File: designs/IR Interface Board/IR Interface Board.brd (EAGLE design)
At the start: 75 x 75 mm, 73 parts, among them IC1 REG1117, IC2 PIC16F1517/19PT

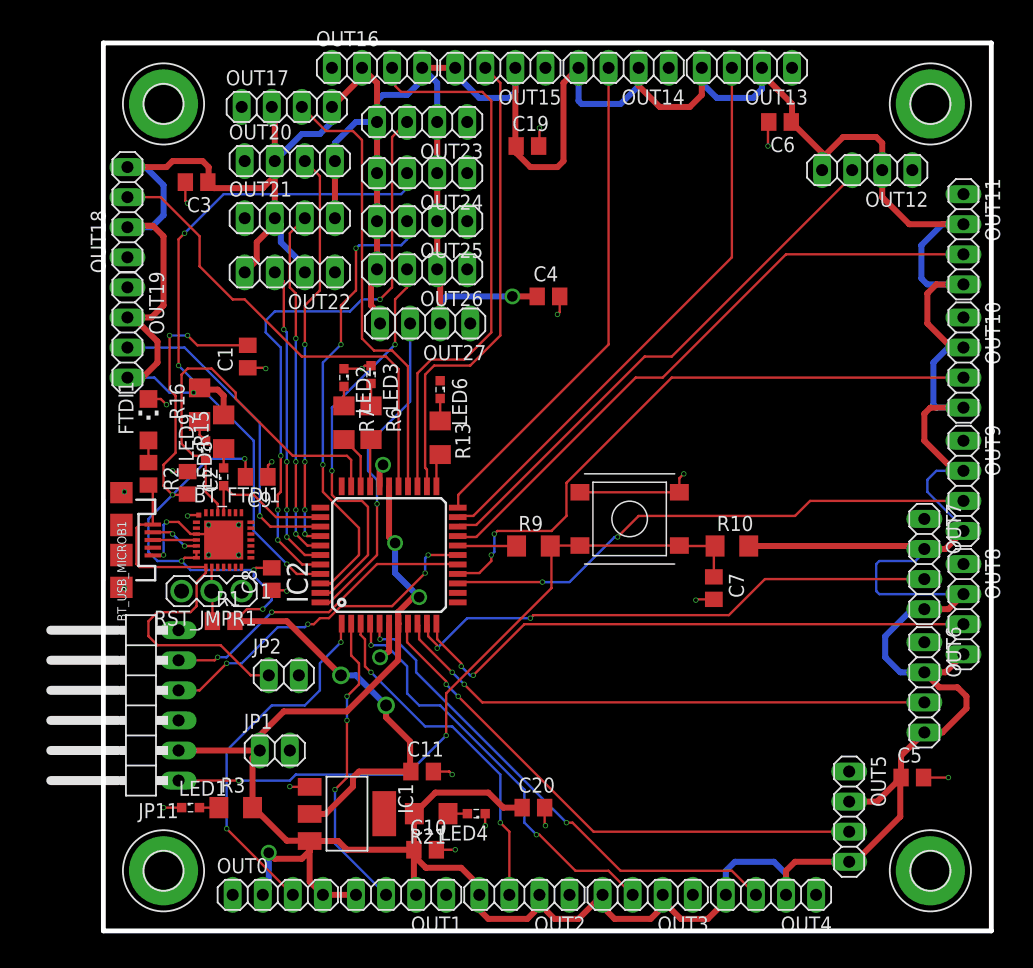
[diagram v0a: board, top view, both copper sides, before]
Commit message: Done with Unknown
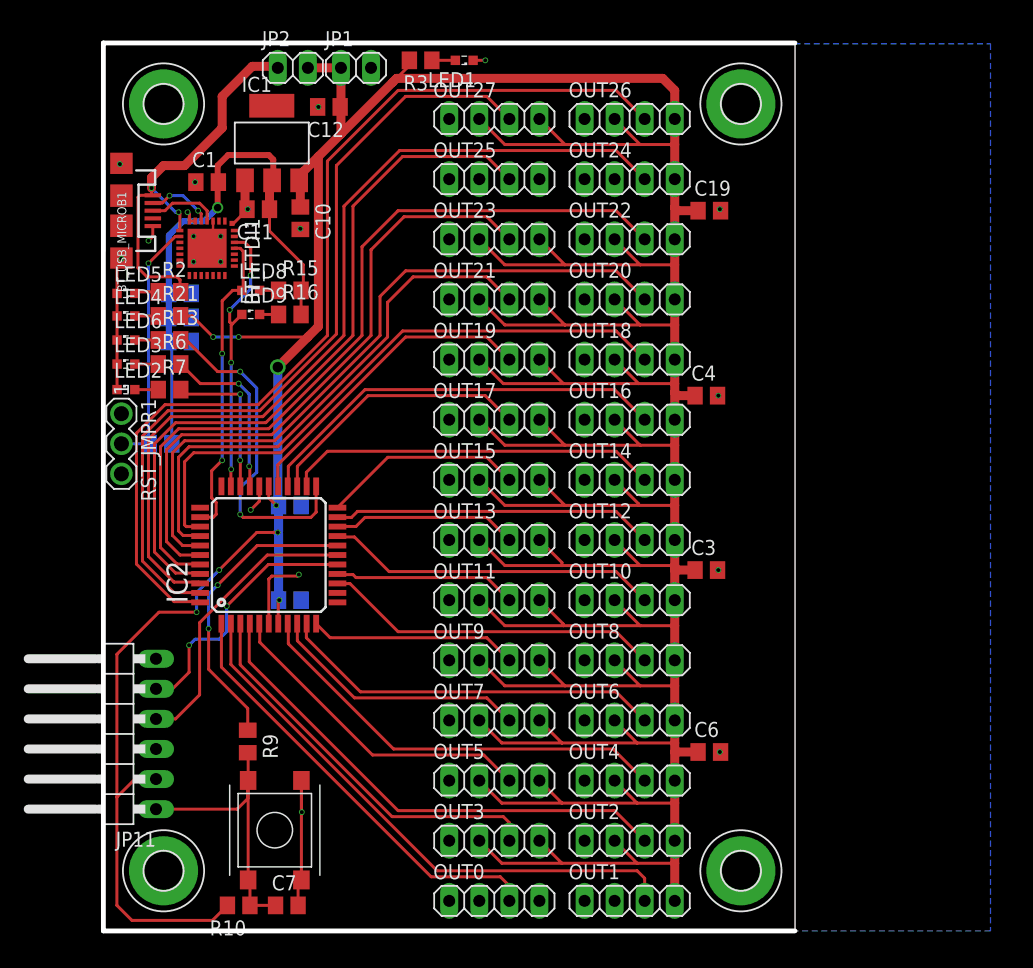
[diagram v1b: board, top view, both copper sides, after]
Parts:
- removed FTDI1: (no value), interface_board-rev13:CHIPLED_1206
- added C12: 10uF, rcl:C0805
- added LED5: (no value), interface_board-rev13:SML0603
- C1, C2, C8, C9: device resistor:C0805 -> rcl:C0805
- C11: value 10uF -> 4.7uF
- C20, C5: value 0.1uF -> 1uF
- C3, C4, C6: value 0.1uF -> 4.7uF
- R10, R13, R15, R16, R21, R3, R6, R7, R9: device rcl:R1206 -> rcl:R0805
- R2: device resistor:R0805 -> rcl:R0805
- moved LED1 67.2 mm to (30.5, 73.5), turned to 180 degrees
- moved R3 65.0 mm to (26.8, 73.5), turned to 180 degrees
- moved JP1 58.1 mm to (21.3, 72.9)
- moved C5 57.4 mm to (15.7, 35.9), flipped to the bottom, turned to 180 degrees
- moved IC1 57.0 mm to (14.2, 66.5), turned to 0 degrees
- moved C10 54.4 mm to (16.6, 60.2), turned to 270 degrees
- moved C3 54.1 mm to (50.9, 30.5), turned to 0 degrees
- moved C6 53.5 mm to (51.2, 15.1), turned to 0 degrees
- moved R10 51.5 mm to (11.4, 2.16), turned to 180 degrees
- moved LED4 51.4 mm to (1.91, 51.9), turned to 0 degrees
- moved JP2 51.3 mm to (16.0, 72.9)
- moved OUT11 50.0 mm to (33.0, 27.9), turned to 0 degrees
- moved C11 49.5 mm to (13.1, 61.0), turned to 180 degrees
- moved R21 47.5 mm to (5.59, 51.9), turned to 0 degrees
- moved OUT13 45.2 mm to (33.0, 33.0), turned to 0 degrees
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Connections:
- removed net GND1: LED6.C
- net +3V3: now also R15.2, R16.2
- net +5V: now also C12.1, JP2.2; no longer R15.2, R16.2
- net ADC_10: now also IC2.11; no longer IC2.14
- net ADC_11: now also IC2.19; no longer IC2.15
- net ADC_12: now also IC2.15; no longer IC2.19
- net ADC_13: now also IC2.21; no longer IC2.20
- net ADC_14: now also IC2.20; no longer IC2.21
- net ADC_15: now also IC2.24; no longer IC2.22
- net ADC_16: now also IC2.22; no longer IC2.24
- net ADC_17: now also IC2.26; no longer IC2.25
- net ADC_18: now also IC2.25; no longer IC2.26
- net ADC_19: now also IC2.36; no longer IC2.27
- net ADC_20: now also IC2.27; no longer IC2.36
- net ADC_21: now also IC2.38; no longer IC2.37
- net ADC_22: now also IC2.37; no longer IC2.38
- net ADC_23: now also IC2.40; no longer IC2.39
- net ADC_24: now also IC2.39; no longer IC2.40
- net ADC_25: now also IC2.42; no longer IC2.41
- net ADC_26: now also IC2.41; no longer IC2.42
- net ADC_27: now also IC2.44; no longer IC2.43
- net ADC_28: now also IC2.43; no longer IC2.44
- net ADC_3: now also IC2.4; no longer IC2.3
- net ADC_4: now also IC2.3; no longer IC2.4
- net ADC_5: now also IC2.8; no longer IC2.5
- net ADC_6: now also IC2.5; no longer IC2.8
- net ADC_7: now also IC2.10; no longer IC2.9
- net ADC_8: now also IC2.9; no longer IC2.10
- net ADC_9: now also IC2.14; no longer IC2.11
- net GND: now also C12.2, LED5.C, LED6.C; no longer FTDI1.C, JP2.2
- net N$12: now also LED5.A; no longer FTDI1.A
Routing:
- net ADC_27: track 34.6 -> 82.3 mm, vias 2 -> 0
- net +3V3: track 89.9 -> 47.5 mm, vias 9 -> 2
- net ADC_23: track 26.2 -> 67.0 mm, vias 4 -> 0
- net ADC_28: track 27.8 -> 68.5 mm, vias 1 -> 0
- net ADC_12: track 52.6 -> 15.4 mm
- net MCLR: track 60.5 -> 24.8 mm, vias 2 -> 0
- net ADC_14: track 48.2 -> 15.6 mm
- net ADC_10: track 45.6 -> 17.6 mm, vias 2 -> 0
- net STATUS_0: track 2.82 -> 28.3 mm, vias 0 -> 2
- net ADC_21: track 33.9 -> 58.9 mm, vias 4 -> 0
- net ADC_11: track 52.4 -> 28.2 mm, vias 2 -> 0
- net ADC_8: track 46.0 -> 22.1 mm, vias 2 -> 0
- net ADC_16: track 40.4 -> 17.1 mm
- net ADC_26: track 38.7 -> 61.0 mm, vias 3 -> 0
- net ADC_2: track 25.8 -> 47.8 mm, vias 3 -> 0
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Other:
- board size 75 x 75 mm -> 58.4 x 75 mm
